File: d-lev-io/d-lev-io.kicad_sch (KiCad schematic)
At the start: 11 parts, among them J1 PJ-059A, J2 USB_C_Receptacle_USB2.0, J8 Conn_01x12, U1 AMS1117-5.0

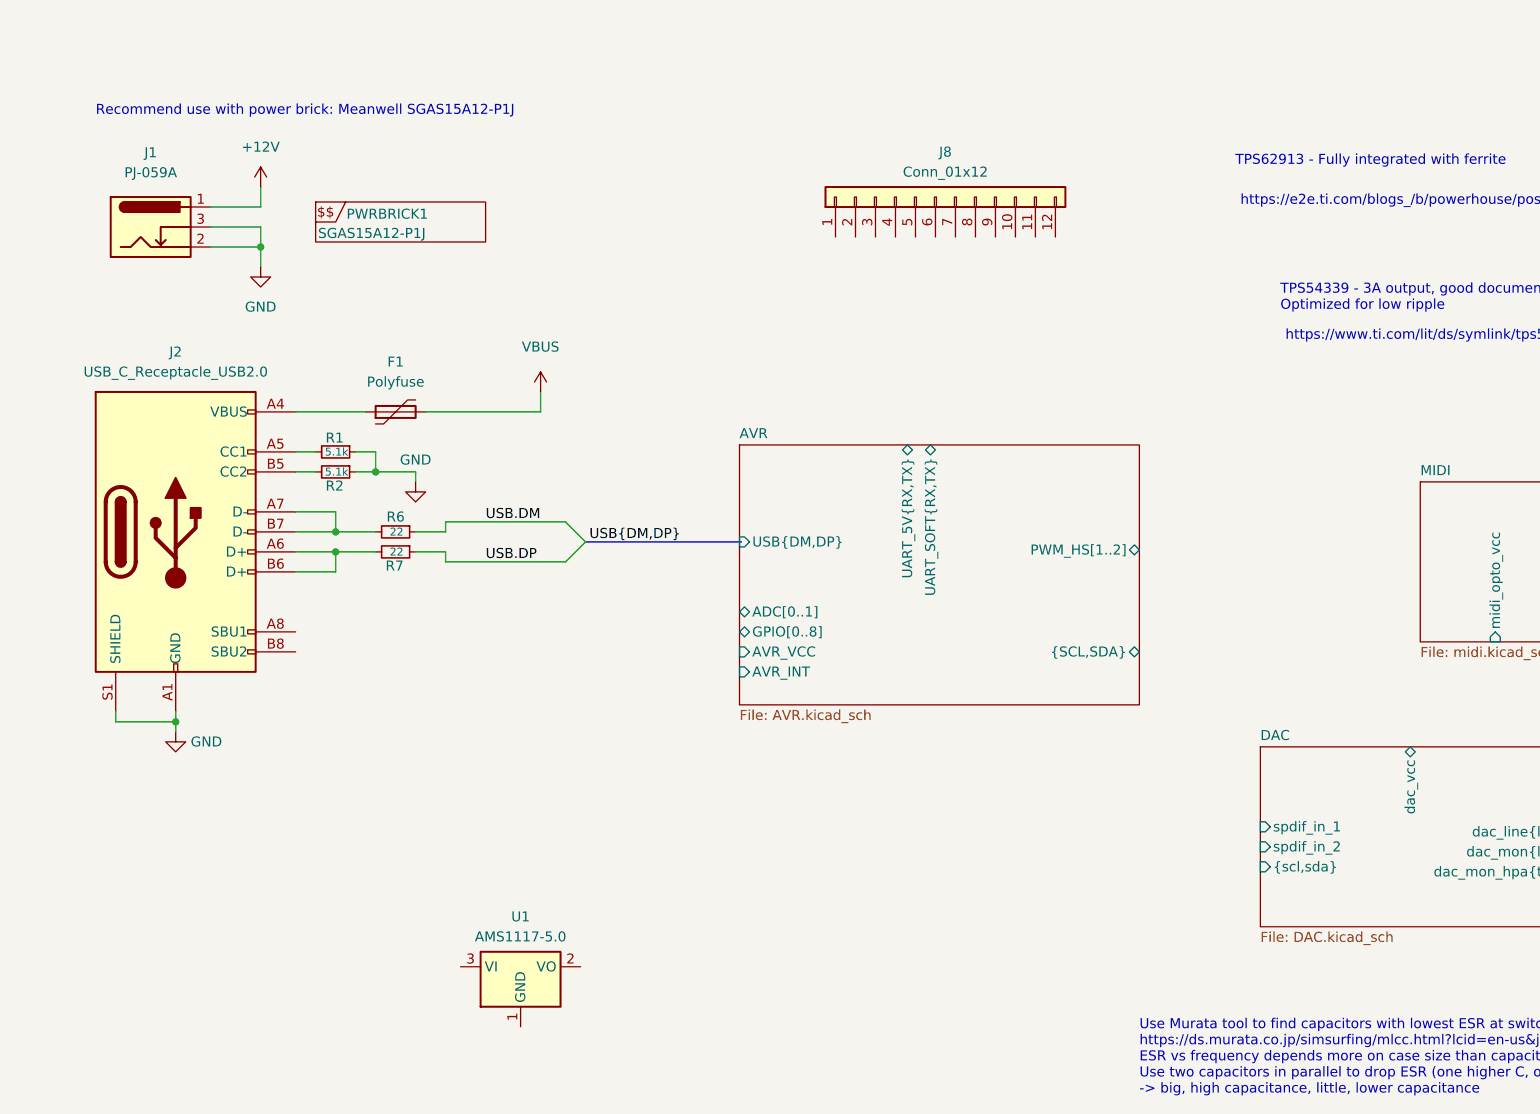
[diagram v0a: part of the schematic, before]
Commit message: more minor pusharounds and updates
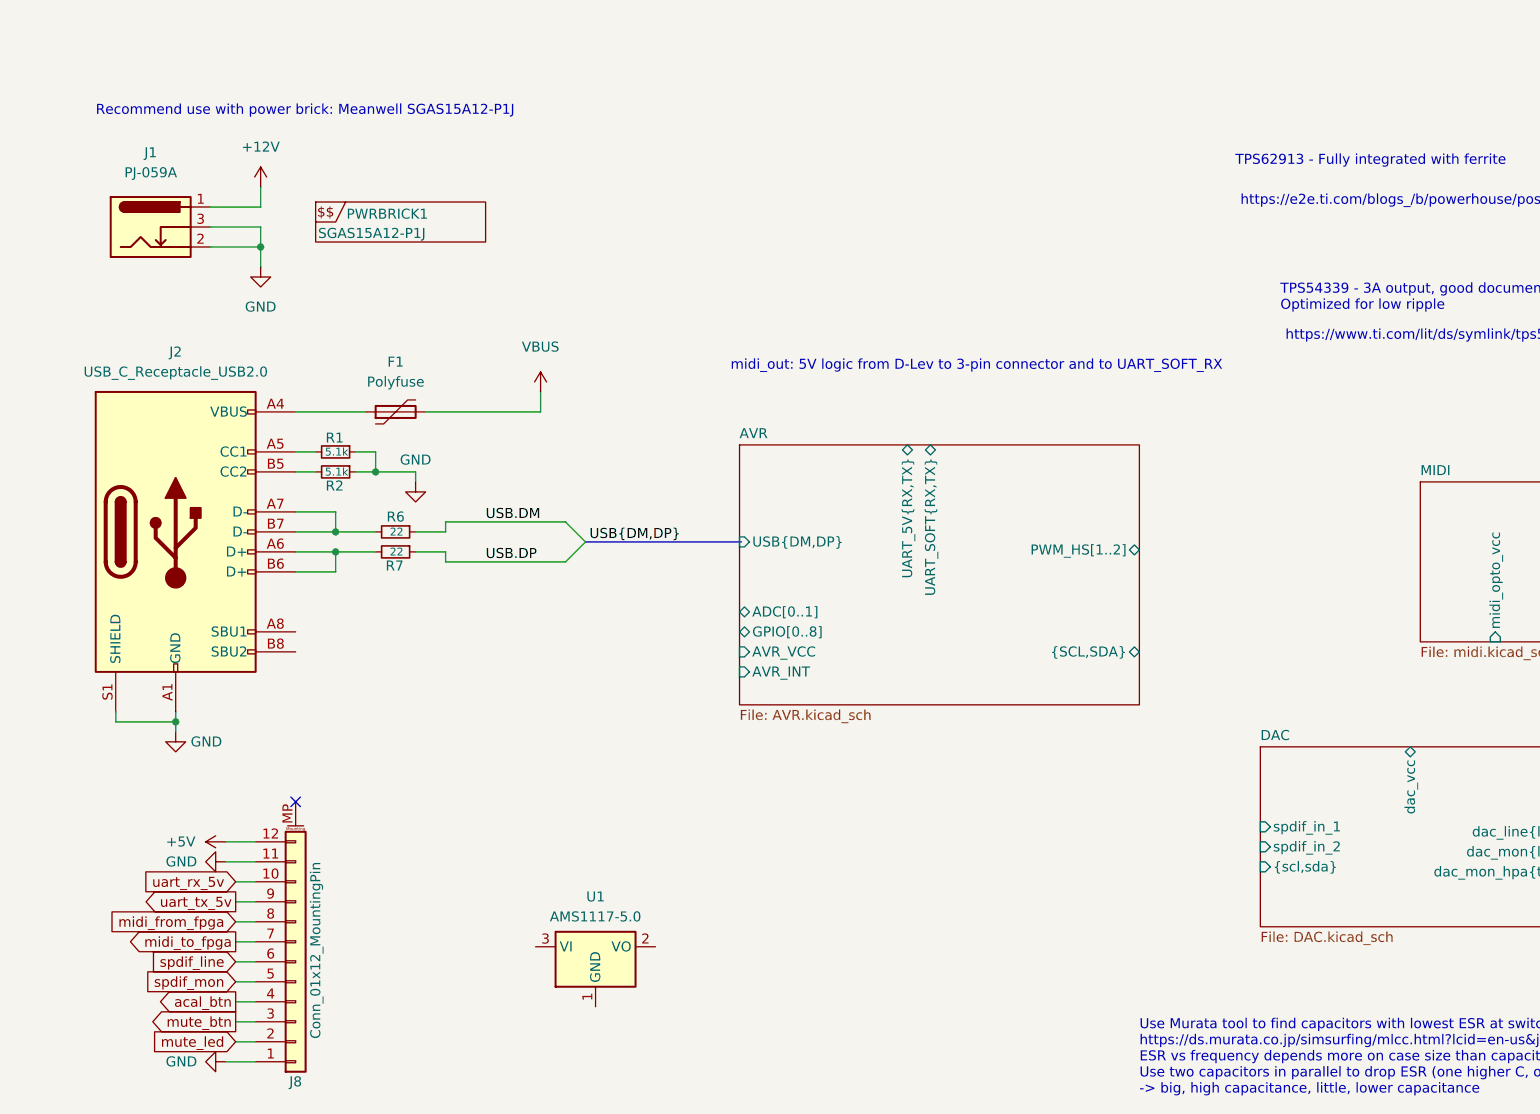
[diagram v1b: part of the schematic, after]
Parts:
- removed J8: Conn_01x12, Connector_JST:JST_PH_S12B-PH-SM4-TB_1x12-1MP_P2.00mm_Horizontal, symbol Connector_Generic:Conn_01x12
- added J8: Conn_01x12_MountingPin, theremin:JST_PH_S12B-PH-SM4-TB_1x12-1MP_P2.00mm_Horizontal, symbol Connector_Generic_MountingPin:Conn_01x12_MountingPin
- J1: footprint (none) -> theremin:BarrelJack_CUI_PJ-059A
- R10: footprint (none) -> Resistor_SMD:R_0603_1608Metric
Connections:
- net +5V: now also J8.12 (Pin_12)
- net GND: now also J8.1 (Pin_1), J8.11 (Pin_11)
- new net acal_btn: J8.4 (Pin_4)
- new net midi_from_fpga: J8.8 (Pin_8)
- new net midi_to_fpga: J8.7 (Pin_7)
- new net mute_btn: J8.3 (Pin_3)
- new net mute_led: J8.2 (Pin_2)
- new net spdif_line: J8.6 (Pin_6)
- new net spdif_mon: J8.5 (Pin_5)
- new net uart_rx_5v: J8.10 (Pin_10)
- new net uart_tx_5v: J8.9 (Pin_9)
- no-connect marks 0 -> 1
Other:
- note added: "midi_out: 5V logic from D-Lev to 3-pin connector and to UART_SOFT_RX"
- moved on the sheet: U1
